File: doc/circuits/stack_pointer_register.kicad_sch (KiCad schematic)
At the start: 5 parts, among them U10 74LS193, U3 74LS245, U4 74LS04, U8 74LS193, U9 74LS245

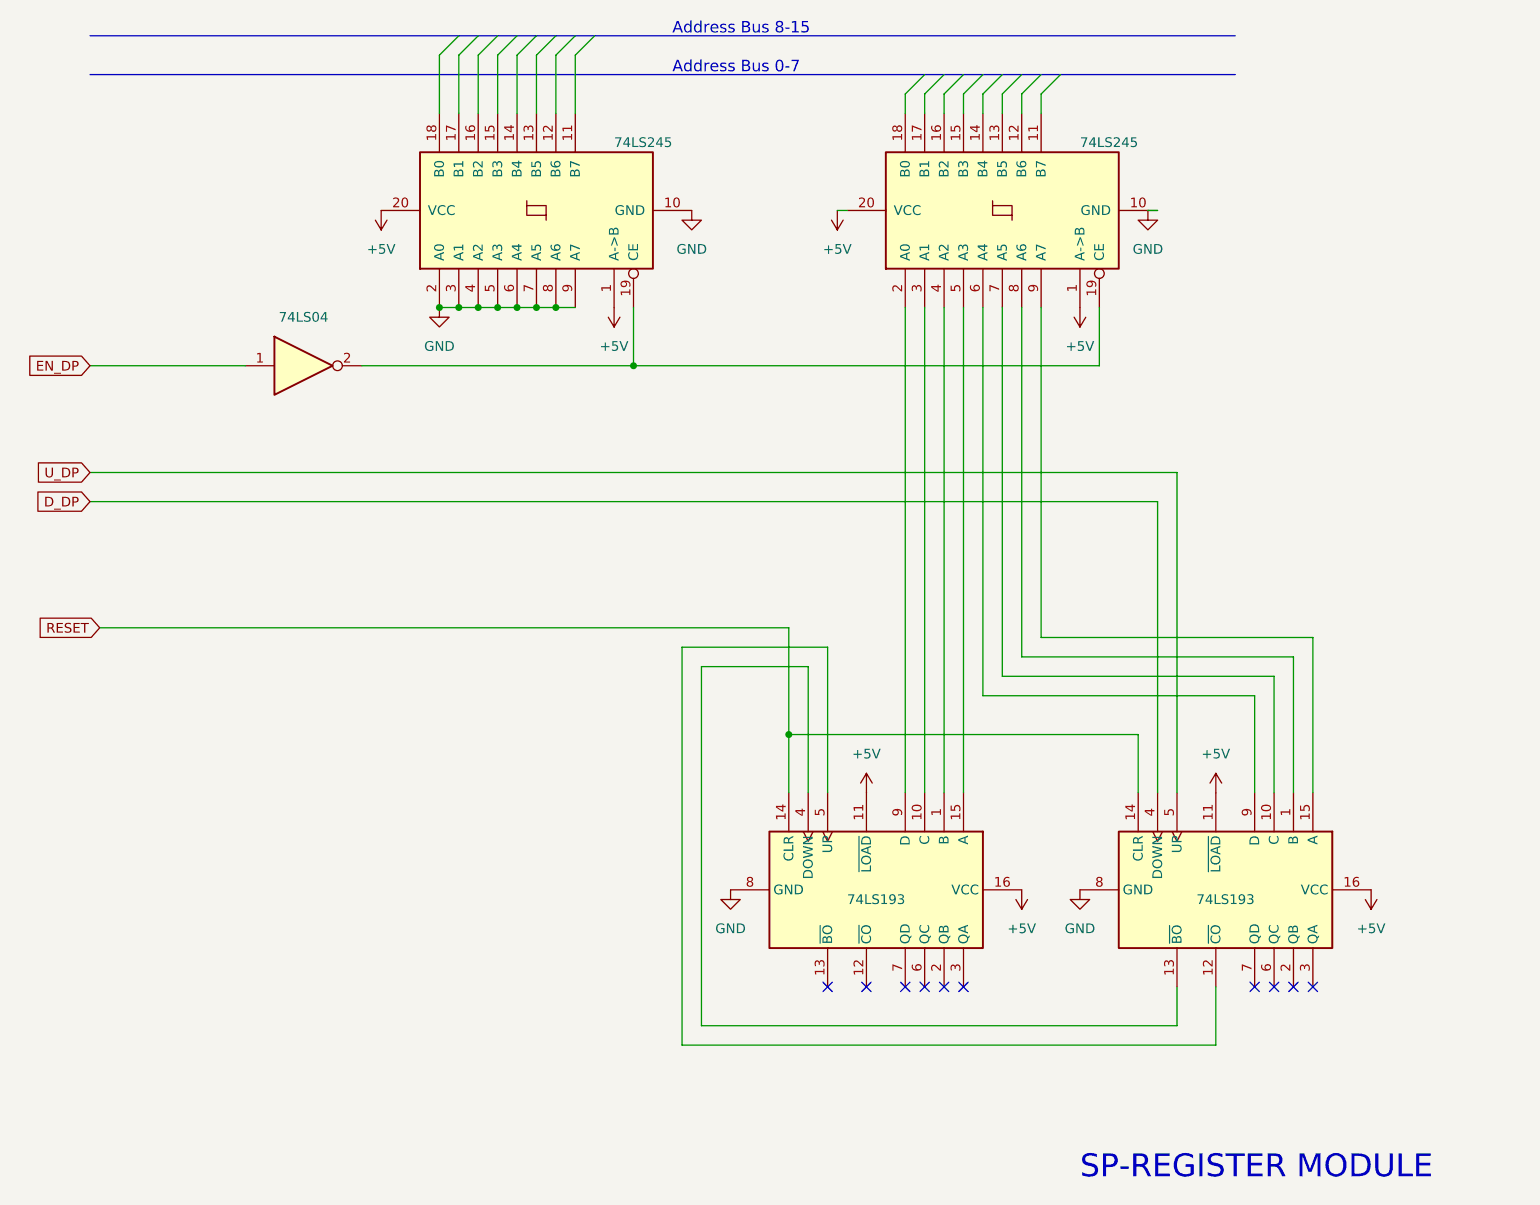
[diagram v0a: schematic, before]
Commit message: Updated schematics
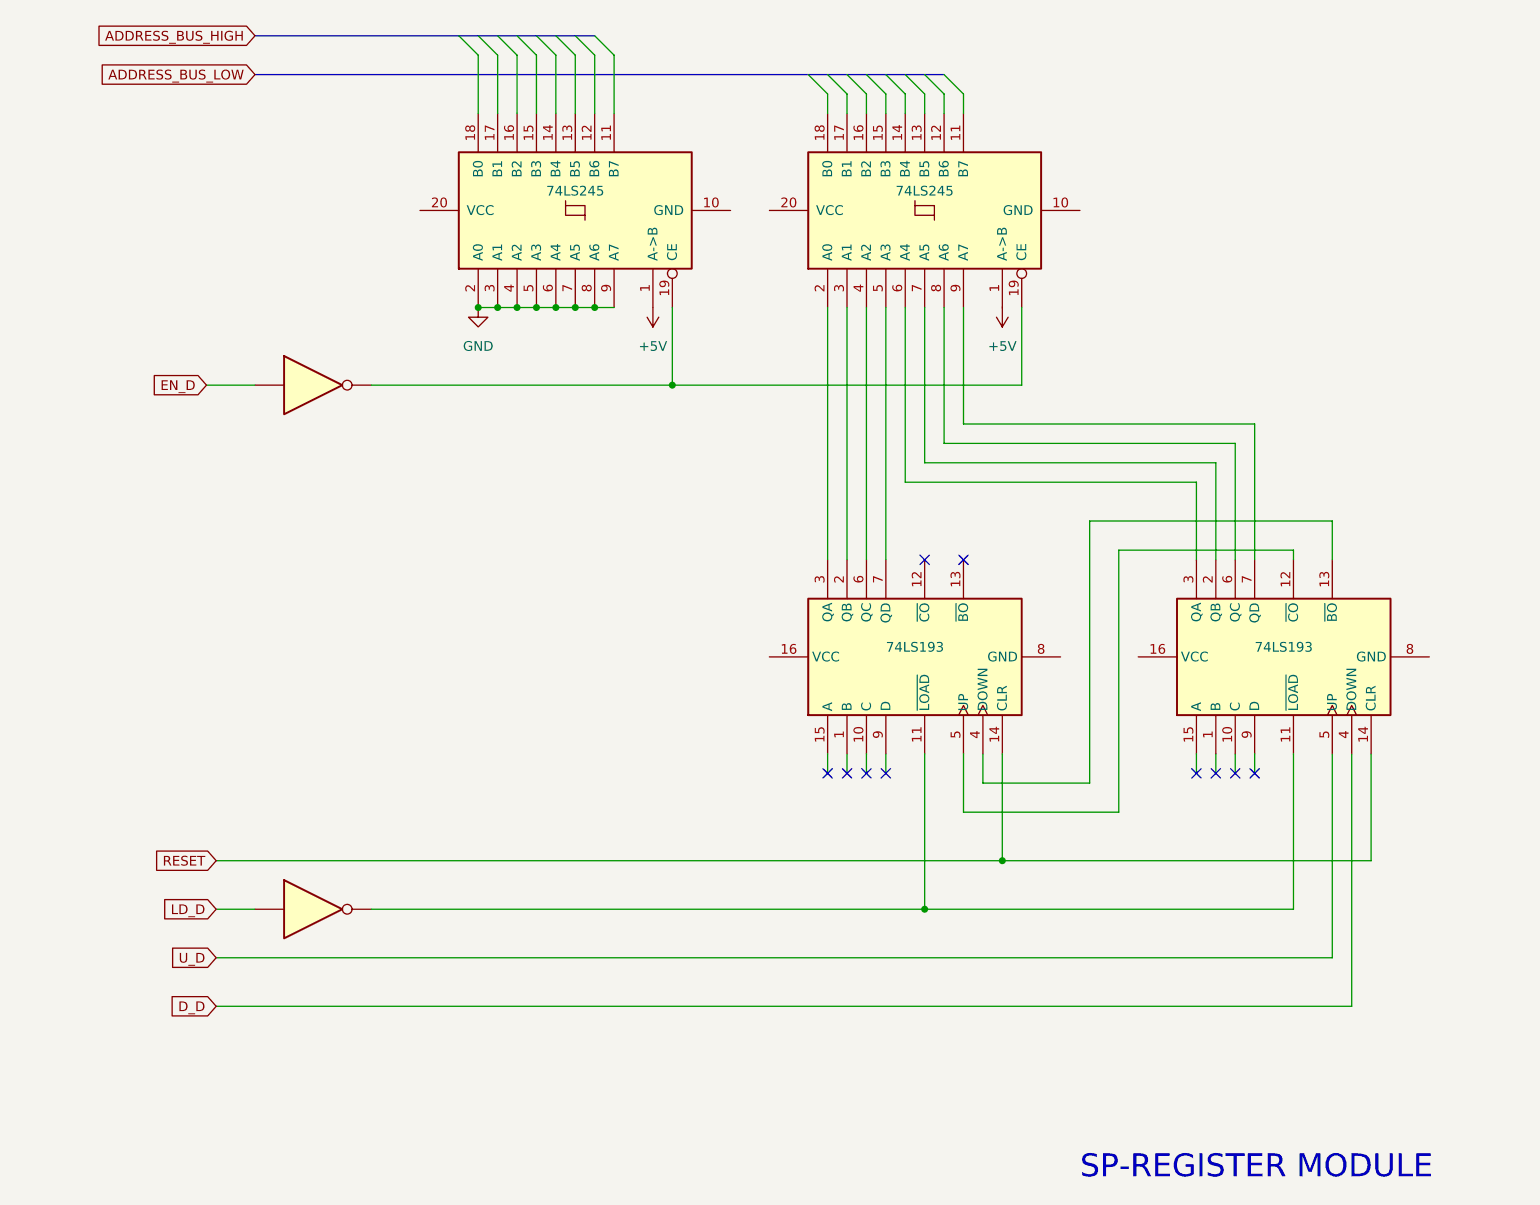
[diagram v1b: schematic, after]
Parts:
- removed U10: 74LS193, symbol 74xx:74LS193
- removed U3, U9: 74LS245, symbol 74xx:74LS245
- removed U4: 74LS04, symbol 74xx:74LS04
- added U1, U7: 74LS245, symbol 74xx:74LS245
- added U2, U5: 74LS04, symbol 74xx:74LS04
- added U6: 74LS193, symbol 74xx:74LS193
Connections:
- net +5V: now also U1.1 (A->B), U7.1 (A->B); no longer U8.11 (~{LOAD}), U8.16 (VCC)
- net GND: now also U1.2 (A0), U1.3 (A1), U1.4 (A2), U1.5 (A3), U1.6 (A4), U1.7 (A5), U1.8 (A6), U1.9 (A7); no longer U8.8 (GND)
- net RESET: now also U6.14 (CLR)
- net at U8.12 (~{CO}): now also U6.5 (UP)
- net at U8.13 (~{BO}): now also U6.4 (DOWN)
- net at U8.2 (QB): now also U7.7 (A5)
- net at U8.3 (QA): now also U7.6 (A4)
- net D_D: now reaches U8.4 (DOWN)
- net U_D: now reaches U8.5 (UP)
- net at U8.6 (QC): now also U7.8 (A6)
- net at U8.7 (QD): now also U7.9 (A7)
- new net: U1.19 (CE), U2.2, U7.19 (CE)
- new net: U6.3 (QA), U7.2 (A0)
- new net: U6.2 (QB), U7.3 (A1)
- new net: U6.6 (QC), U7.4 (A2)
- new net: U6.7 (QD), U7.5 (A3)
- new net: U5.2, U6.11 (~{LOAD}), U8.11 (~{LOAD})
- new net EN_D: U2.1
- new net LD_D: U5.1
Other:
- note removed: "Address Bus 0-7"
- note removed: "Address Bus 8-15"
